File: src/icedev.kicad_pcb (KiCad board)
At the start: 4 copper layers, 35.6 x 50.8 mm, 52 parts, among them J1 Conn_01x08, J11 USB_C_Receptacle_PowerOnly_6P, J2 Conn_02x01, J3 Conn_01x16, J4 Conn_02x01, J5 Conn_02x01, J6 Conn_01x16, J7 Conn_02x02_Odd_Even, J8 Conn_01x03, J9 Conn_02x01, U1 ICE40UP5K-SG48ITR, U2 AMS1117-1.2, U3 AMS1117-3.3, U4 W25Q128JVS, U5 FM24C64B, X1 MPUOSC

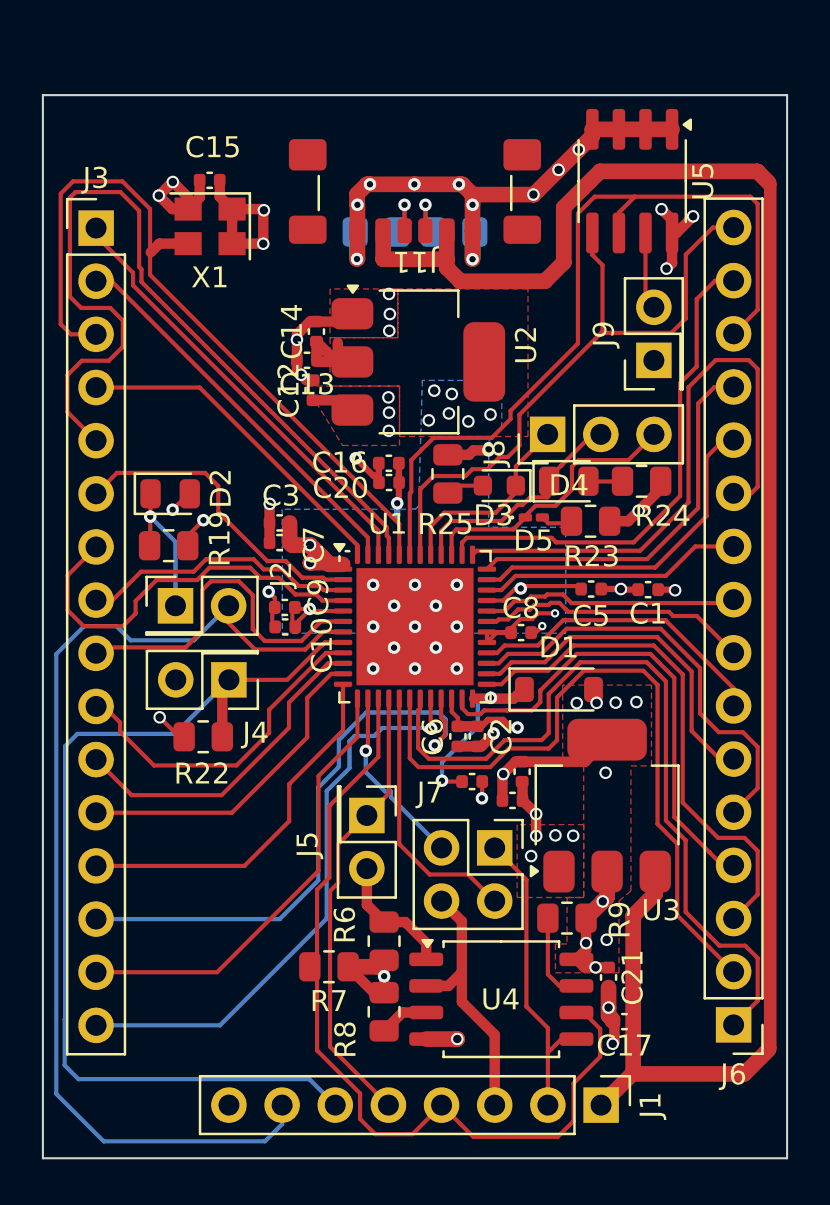
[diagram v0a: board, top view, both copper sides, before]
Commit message: Rev 2
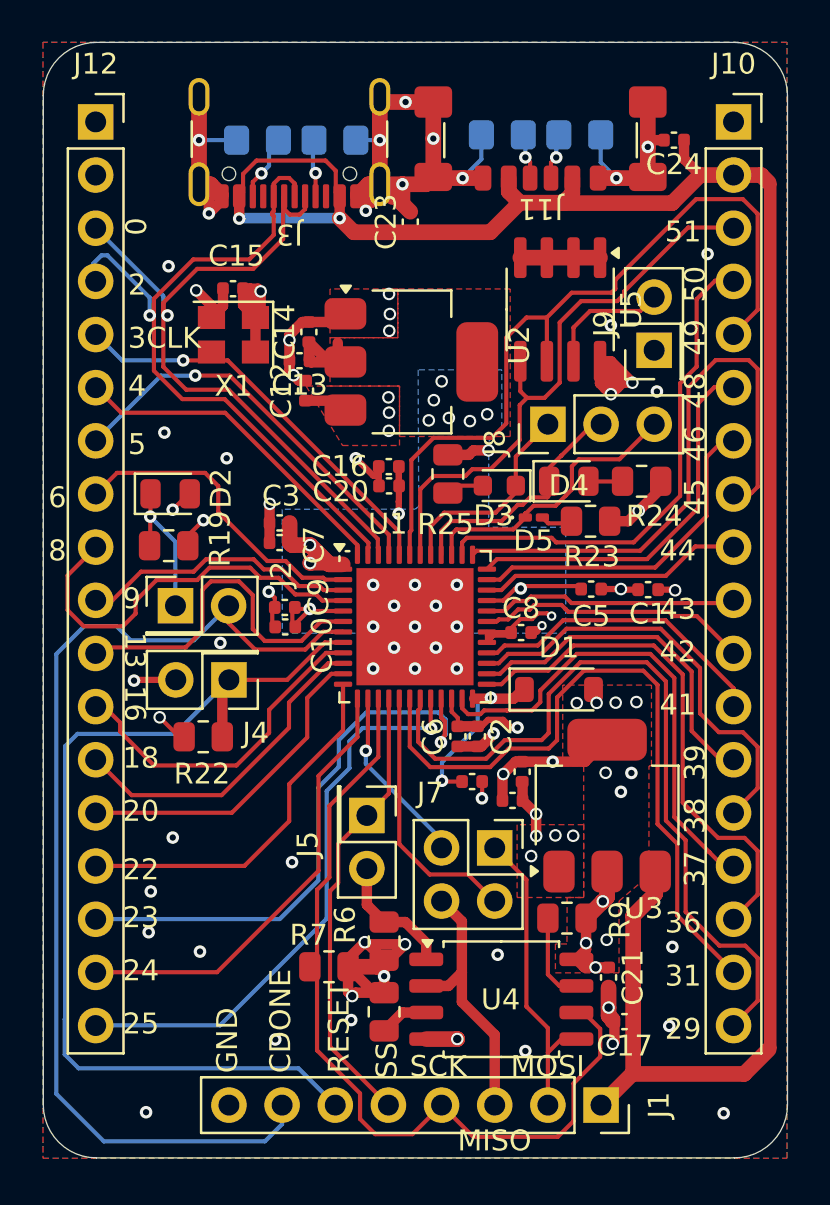
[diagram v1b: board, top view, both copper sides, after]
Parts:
- removed J6: Conn_01x16, Connector_PinHeader_2.54mm:PinHeader_1x16_P2.54mm_Vertical
- added C23: 0.1u, Capacitor_SMD:C_0402_1005Metric, F.Cu at (159.8, 90.7)
- added C24: 0.1u, Capacitor_SMD:C_0402_1005Metric, F.Cu at (172.4, 86.8)
- added J10: Conn_01x18, Connector_PinSocket_2.54mm:PinSocket_1x18_P2.54mm_Vertical, F.Cu at (175.2, 85.9)
- added J12: Conn_01x18, Connector_PinSocket_2.54mm:PinSocket_1x18_P2.54mm_Vertical, F.Cu at (144.7, 85.9)
- added R26: 5.1K, Resistor_SMD:R_0805_2012Metric_Pad1.20x1.40mm_HandSolder, B.Cu at (156.2, 86.8)
- added R27: 5.1K, Resistor_SMD:R_0805_2012Metric_Pad1.20x1.40mm_HandSolder, B.Cu at (152.5, 86.8)
- D1: value MBR130 -> Schottky Diode
- J1: footprint Connector_PinHeader_2.54mm:PinHeader_1x08_P2.54mm_Vertical -> Connector_PinSocket_2.54mm:PinSocket_1x08_P2.54mm_Vertical
- J3: value Conn_01x16 -> USB_C_Receptacle_USB2.0_14P; footprint Connector_PinHeader_2.54mm:PinHeader_1x16_P2.54mm_Vertical -> Connector_USB:USB_C_Receptacle_GCT_USB4105-xx-A_16P_TopMnt_Horizontal
- moved J3 10.6 mm to (154.0, 85.8), turned to 180 degrees
- moved R21 7.61 mm to (164.2, 86.5)
- moved R20 7.60 mm to (167.9, 86.5)
- moved U5 7.03 mm to (166.9, 94.8)
- moved J11 6.51 mm to (166.0, 85.5)
- moved C15 5.30 mm to (151.3, 93.8)
- moved X1 5.30 mm to (151.3, 96.0)
- moved J9 0.49 mm to (171.4, 96.8)
- moved J8 0.49 mm to (166.4, 100.3)
- moved C13 0.36 mm to (154.5, 97.3)
- moved C12 0.36 mm to (154.8, 98.7)
- moved C14 0.36 mm to (154.9, 95.9)
- moved U2 0.34 mm to (159.8, 97.3)
- moved C16 0.16 mm to (158.8, 102.3)
- moved C20 0.16 mm to (158.8, 103.3)
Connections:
- J11 pad S1: unconnected-(J11-SHIELD-PadS1) -> GND
- U1 pad 46: IO0 -> D-
- U1 pad 47: IO2 -> D+
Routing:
- net D-: track 0.00 -> 35.2 mm, vias 0 -> 1
- net D+: track 0.00 -> 35.1 mm, vias 0 -> 1
- net GND: track 57.1 -> 81.2 mm, vias 46 -> 66
- net IO5: track 41.1 -> 19.4 mm, vias 0 -> 1
- net IO0: track 21.2 -> 0.00 mm
- net IO2: track 18.9 -> 0.00 mm
- net CLK: track 36.6 -> 19.5 mm, vias 0 -> 1
- net +5V: track 86.5 -> 101.8 mm, vias 0 -> 2
- net +3V3: track 57.9 -> 69.8 mm, vias 28 -> 32
- net Net-(J3-CC2): track 0.00 -> 3.19 mm, vias 0 -> 1
- net IO51: track 30.9 -> 27.9 mm
- net Net-(J3-CC1): track 0.00 -> 2.76 mm, vias 0 -> 1
- net Net-(J9-Pin_2): track 3.72 -> 6.07 mm
- net IO49: track 39.1 -> 37.5 mm
- net +1V2: track 18.7 -> 20.1 mm
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- added copper zone on In2.Cu, net +3V3
- added copper zone on B.Cu, net GND
- added copper zone on In1.Cu, net GND
- removed copper zone on In1.Cu, net +3V3
- removed copper zone on In2.Cu, net GND
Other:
- board size 35.6 x 50.8 mm -> 35.6 x 53.3 mm
- board text added: "0"
- board text added: "13"
- board text added: "16"
- board text added: "18"
- board text added: "2"
- board text added: "20"
- board text added: "22"
- board text added: "23"
- board text added: "24"
- board text added: "25"
- board text added: "29"
- board text added: "31"
- board text added: "36"
- board text added: "37"
- board text added: "38"
- board text added: "39"
- board text added: "3CLK"
- board text added: "4"
- board text added: "41"
- board text added: "42"
- board text added: "43"
- board text added: "44"
- board text added: "45"
- board text added: "46"
- board text added: "48"
- board text added: "49"
- board text added: "5"
- board text added: "50"
- board text added: "51"
- board text added: "6"
- board text added: "8"
- board text added: "9"
- board text added: "CDONE"
- board text added: "GND"
- board text added: "MISO"
- board text added: "MOSI"
- board text added: "RESET"
- board text added: "SCK"
- board text added: "SS"
